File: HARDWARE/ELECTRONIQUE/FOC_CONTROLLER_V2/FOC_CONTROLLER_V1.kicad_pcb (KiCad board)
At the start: 8 copper layers, 50 x 43.3 mm, 0 parts

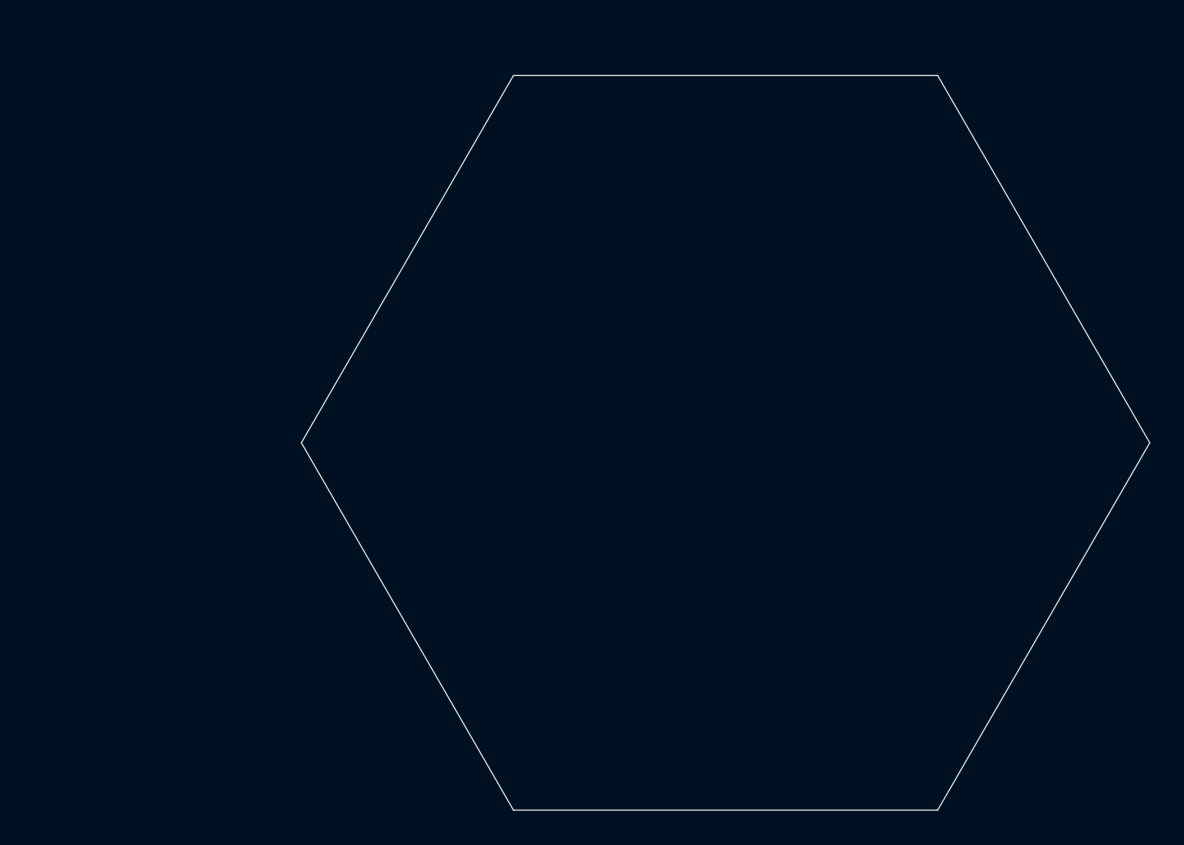
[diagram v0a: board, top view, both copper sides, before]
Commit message: up
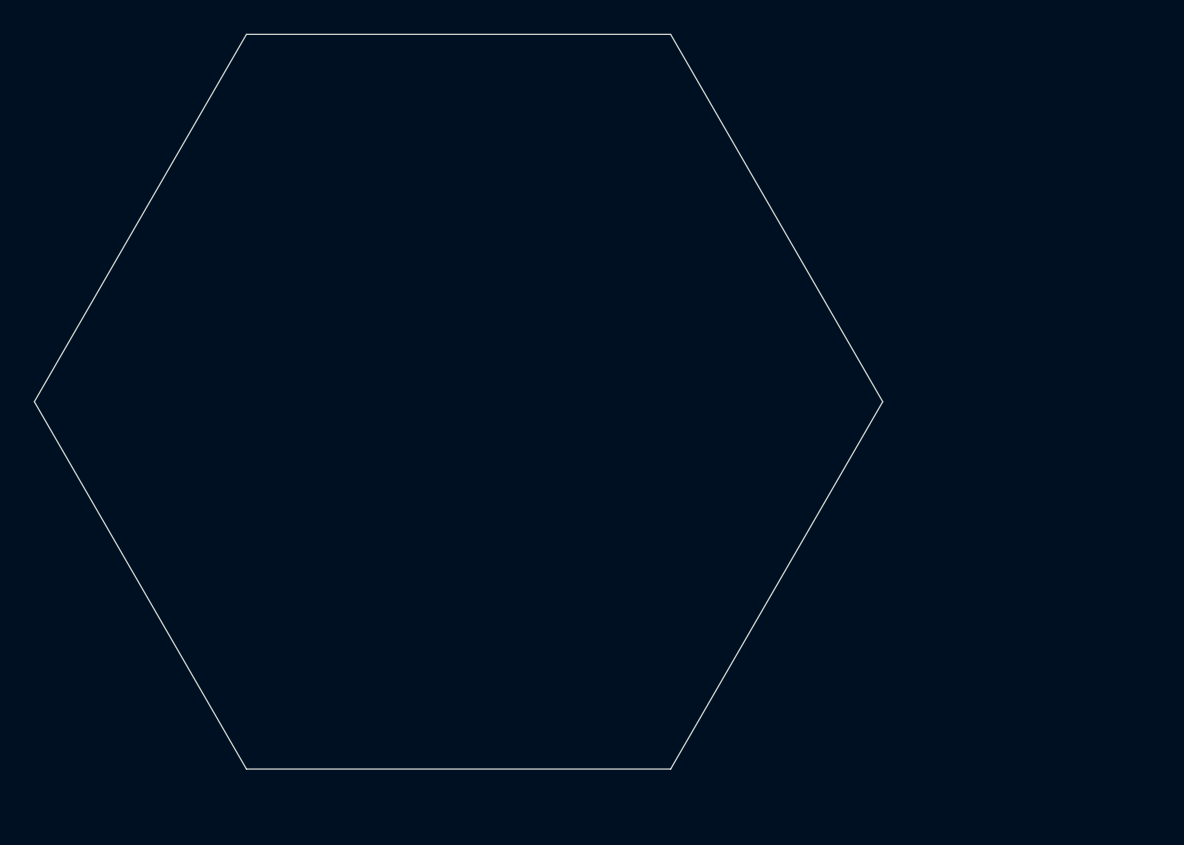
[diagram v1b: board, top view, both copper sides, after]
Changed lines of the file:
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@@
 	(net 0 "")
 	(gr_line
-		(start 150 98.2)
-		(end 170.091472 63.395076)
+		(start 134.262316 95.777737)
+		(end 154.353788 60.972813)
 		(stroke
 			(width 0.1)
@@
 	)
 	(gr_line
-		(start 150 98.2)
-		(end 170.096211 133.002187)
+		(start 134.262316 95.777737)
+		(end 154.358527 130.579924)
 		(stroke
 			(width 0.1)
@@
 	)
 	(gr_arc
-		(start 170.091472 63.395076)
-		(mid 190.187684 98.197263)
-		(end 170.096212 133.002187)
+		(start 154.353788 60.972813)
+		(mid 174.45 95.775)
+		(end 154.358528 130.579924)
 		(stroke
 			(width 0.1)
@@
 	)
 	(gr_arc
-		(start 170.096212 133.002186)
-		(mid 129.907344 133.004239)
-		(end 109.812317 98.2)
+		(start 154.358528 130.579923)
+		(mid 114.16966 130.581976)
+		(end 94.074633 95.777737)
 		(stroke
 			(width 0.1)
@@
 	)
 	(gr_line
-		(start 109.812317 98.2)
-		(end 150 98.2)
+		(start 94.074633 95.777737)
+		(end 134.262316 95.777737)
 		(stroke
 			(width 0.1)
@@
 	)
 	(gr_arc
-		(start 109.812316 98.2)
-		(mid 129.904973 63.397129)
-		(end 170.091472 63.395077)
+		(start 94.074632 95.777737)
+		(mid 114.167289 60.974866)
+		(end 154.353788 60.972814)
 		(stroke
 			(width 0.1)
@@
 	)
 	(gr_rect
-		(start 125 73.2)
-		(end 175 123.2)
+		(start 109.262316 70.777737)
+		(end 159.262316 120.777737)
 		(stroke
 			(width 0.1)
@@
 	(gr_poly
 		(pts
-			(xy 175 98.2) (xy 162.5 119.85) (xy 137.5 119.85) (xy 125 98.2) (xy 137.5 76.55) (xy 162.5 76.55)
+			(xy 159.262316 95.777737) (xy 146.762316 117.427737) (xy 121.762316 117.427737) (xy 109.262316 95.777737)
+			(xy 121.762316 74.127737) (xy 146.762316 74.127737)
 		)
 		(stroke
